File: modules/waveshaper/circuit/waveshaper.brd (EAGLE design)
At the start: 100 x 80 mm, 5 parts, among them IC2 LM324N

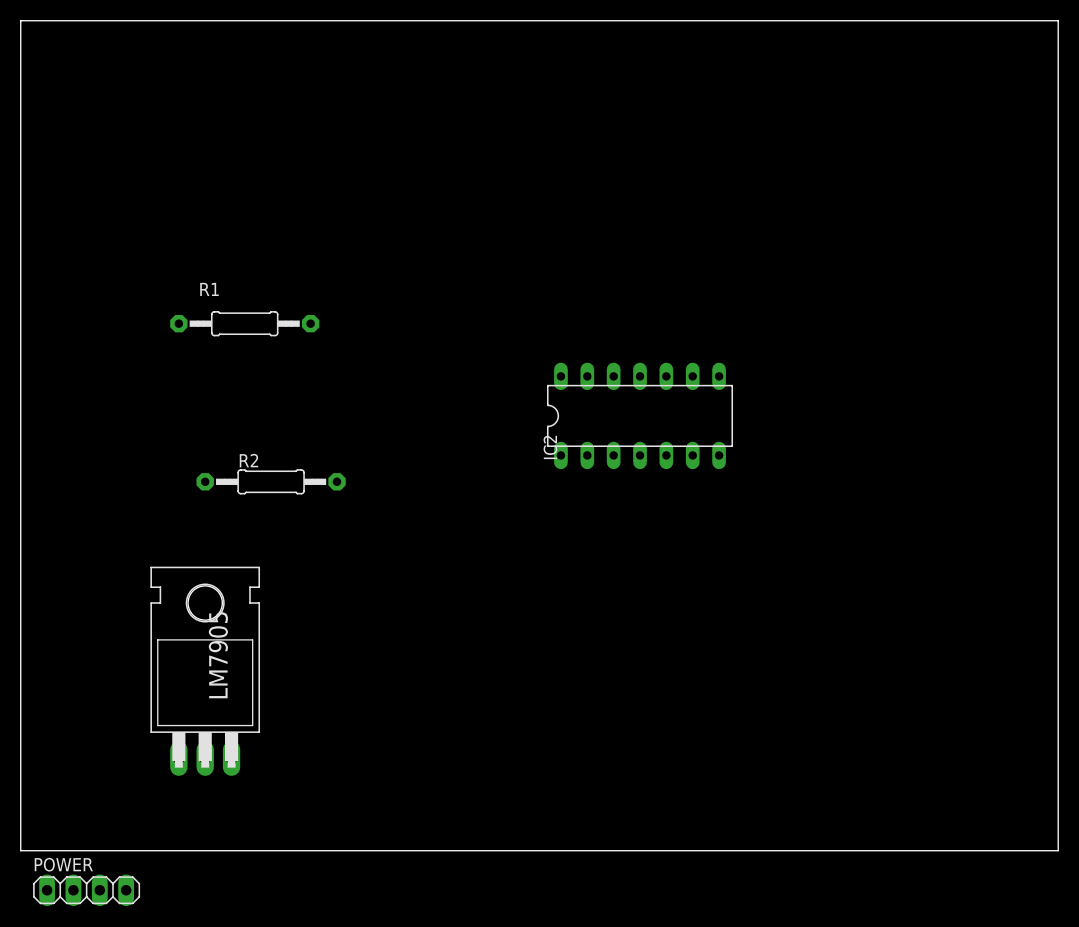
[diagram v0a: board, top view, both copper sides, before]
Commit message: Cleanup
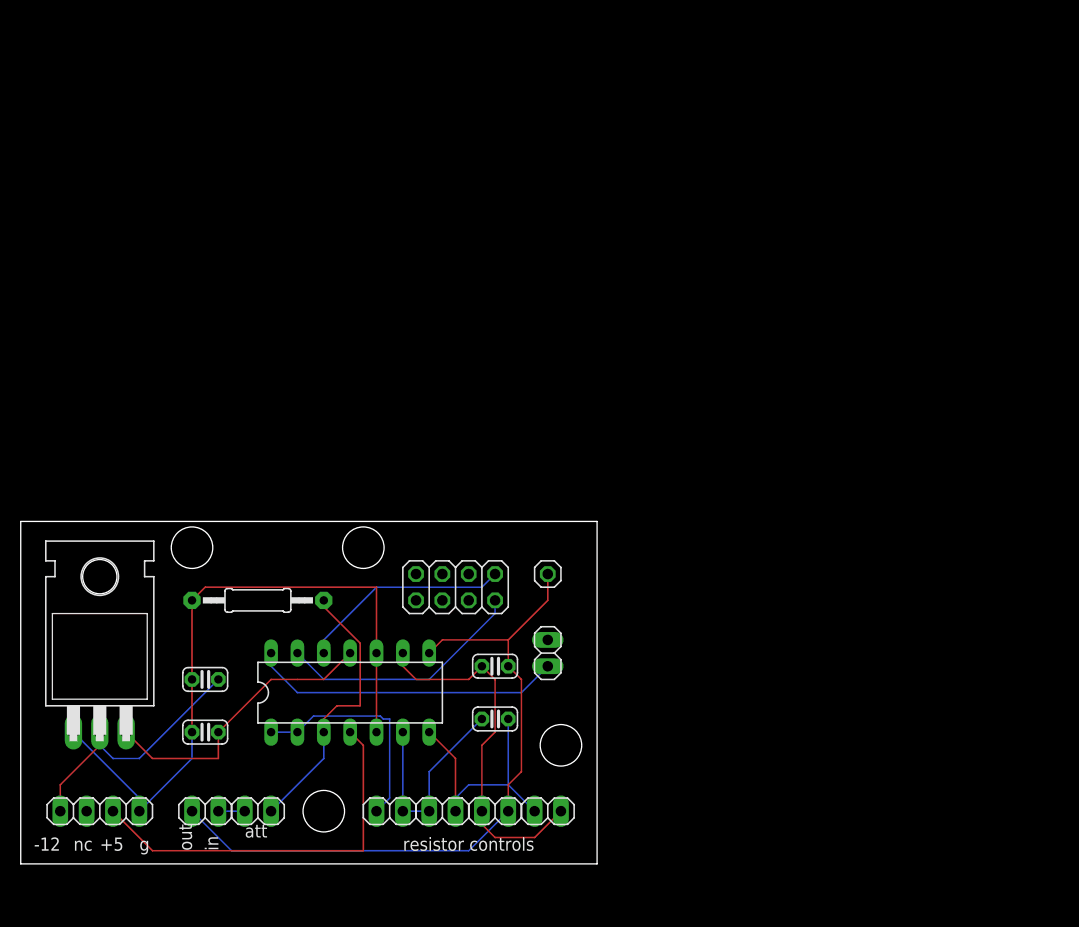
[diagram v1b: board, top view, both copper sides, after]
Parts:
- removed R2: (no value), adafruit:0207/12
- added ATTENUATION, OPTOUT, POTS, POTS1, POTS2, POTS3, SIGNAL: (no value), pinhead:1X02
- added C1: 100uf, adafruit:C025-024X044
- added C2: 0.1uf, adafruit:C025-024X044
- added C3, C4: 33uf, adafruit:C025-024X044
- added JP1: (no value), pinhead:2X04
- added JP2: (no value), pinhead:1X01
- R1: value (none) -> 1K
- moved IC2 38.6 mm to (31.8, 15.2)
- moved R1 26.7 mm to (22.9, 24.1), turned to 180 degrees
- moved LM7905 10.5 mm to (7.62, 21.6)
- moved POWER 7.73 mm to (7.62, 3.81)
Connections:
- removed net 3.3V: LM7905.1, POWER.4
- removed net VDD: IC2.11, IC2.4, LM7905.2, LM7905.3, POWER.1, POWER.2, POWER.3
- new net -12V: C1.2, LM7905.2, POWER.1
- new net -5V: C2.2, IC2.11, LM7905.3
- new net 12V: POWER.2
- new net 5V: IC2.4, POWER.3
- new net GND: C1.1, C2.1, IC2.10, IC2.5, LM7905.1, POWER.4, R1.2
- new net IN: ATTENUATION.2, IC2.3, R1.1
- new net N$1: ATTENUATION.1, SIGNAL.2
- new net N$2: C3.1, IC2.6, POTS.2, POTS1.1
- new net N$3: C3.2, IC2.7, POTS1.2, POTS3.1
- new net N$4: C4.1, IC2.9, POTS2.1, POTS3.2
- new net N$5: IC2.14, OPTOUT.1
- new net N$6: IC2.13, JP1.2
- new net N$7: IC2.12, JP1.1
- new net N$8: IC2.1, IC2.2, POTS.1
- new net OUT: C4.2, IC2.8, JP2.1, POTS2.2, SIGNAL.1
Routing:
- net OUT: track 0.00 -> 67.3 mm
- net GND: track 0.00 -> 66.2 mm
- net 5V: track 0.00 -> 37.7 mm
- net N$4: track 0.00 -> 35.4 mm
- net N$5: track 0.00 -> 30.0 mm
- net -5V: track 0.00 -> 28.3 mm
- net IN: track 0.00 -> 26.6 mm
- net -12V: track 0.00 -> 25.6 mm
- net N$3: track 0.00 -> 25.5 mm
- net N$6: track 0.00 -> 24.0 mm
- net N$8: track 0.00 -> 21.6 mm
- net N$2: track 0.00 -> 21.2 mm
- net N$7: track 0.00 -> 20.4 mm
- net N$1: track 0.00 -> 2.54 mm
- net 12V: track 0.00 -> 1.27 mm
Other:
- board size 100 x 80 mm -> 55.5 x 33 mm
- board text added: "+5"
- board text added: "-12"
- board text added: "att"
- board text added: "g"
- board text added: "in"
- board text added: "nc"
- board text added: "out"
- board text added: "resistor controls"
